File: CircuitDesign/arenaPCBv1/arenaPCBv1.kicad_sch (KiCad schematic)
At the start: 17 parts, among them Q1 IRF520N

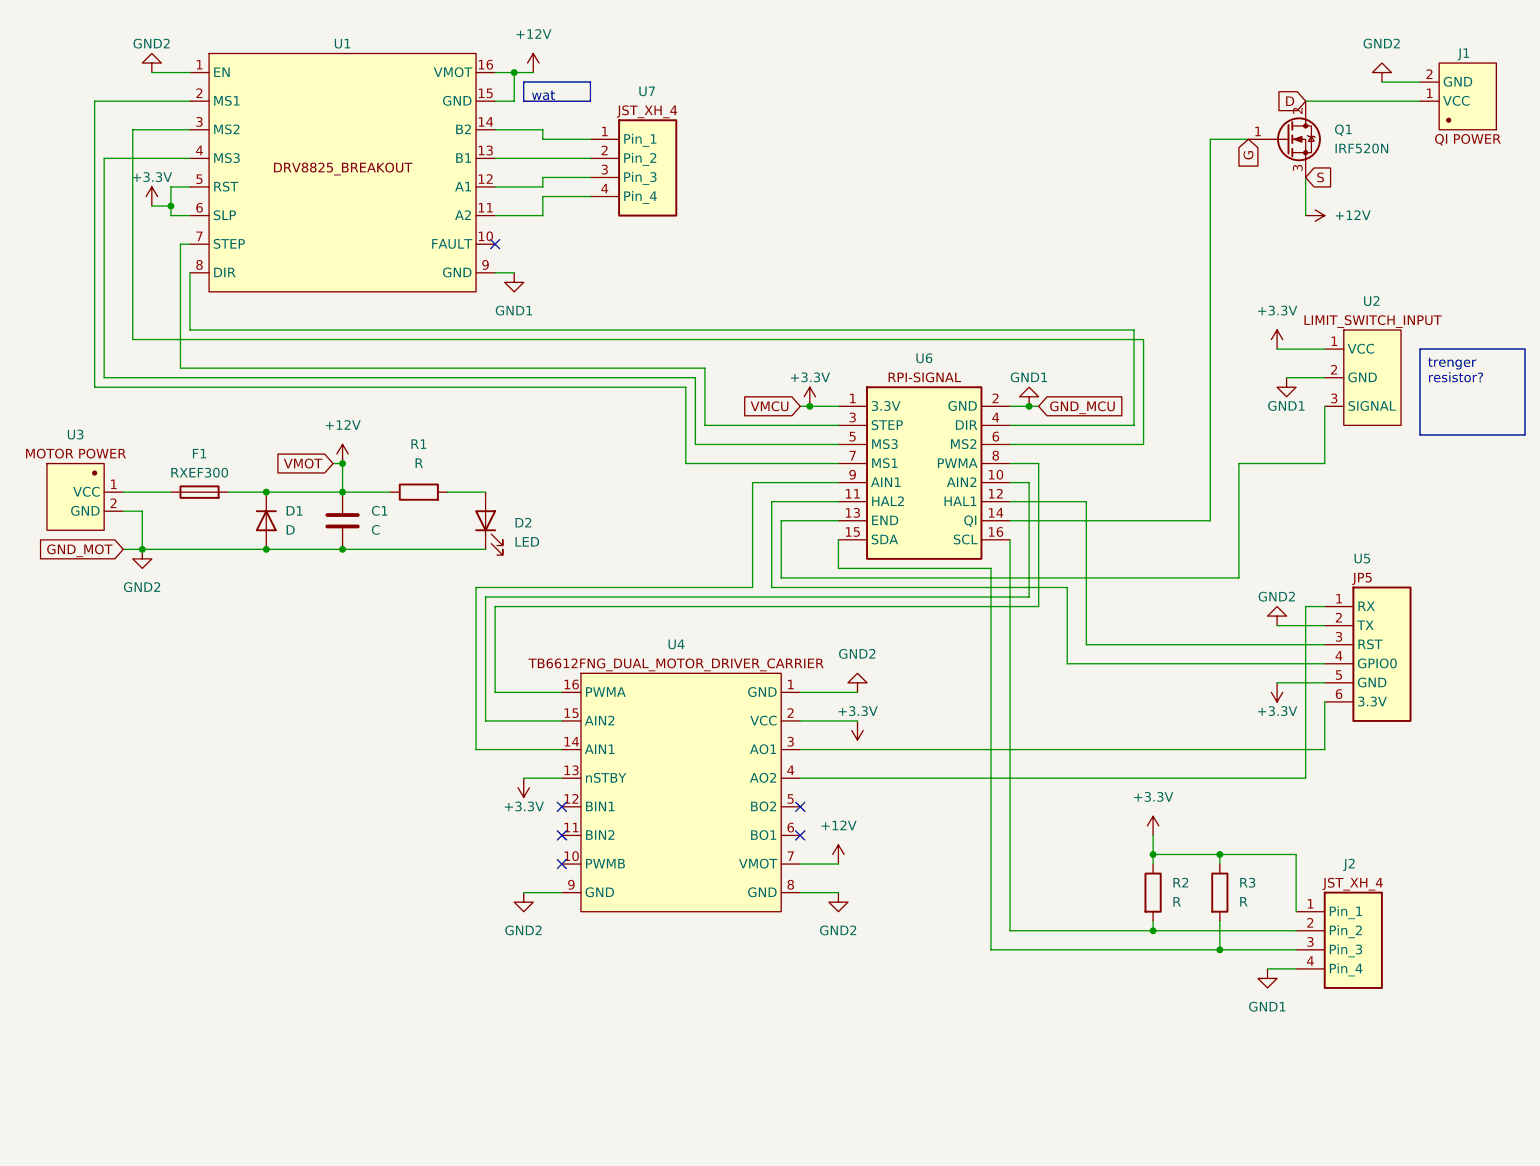
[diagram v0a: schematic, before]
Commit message: PCB v1 finished
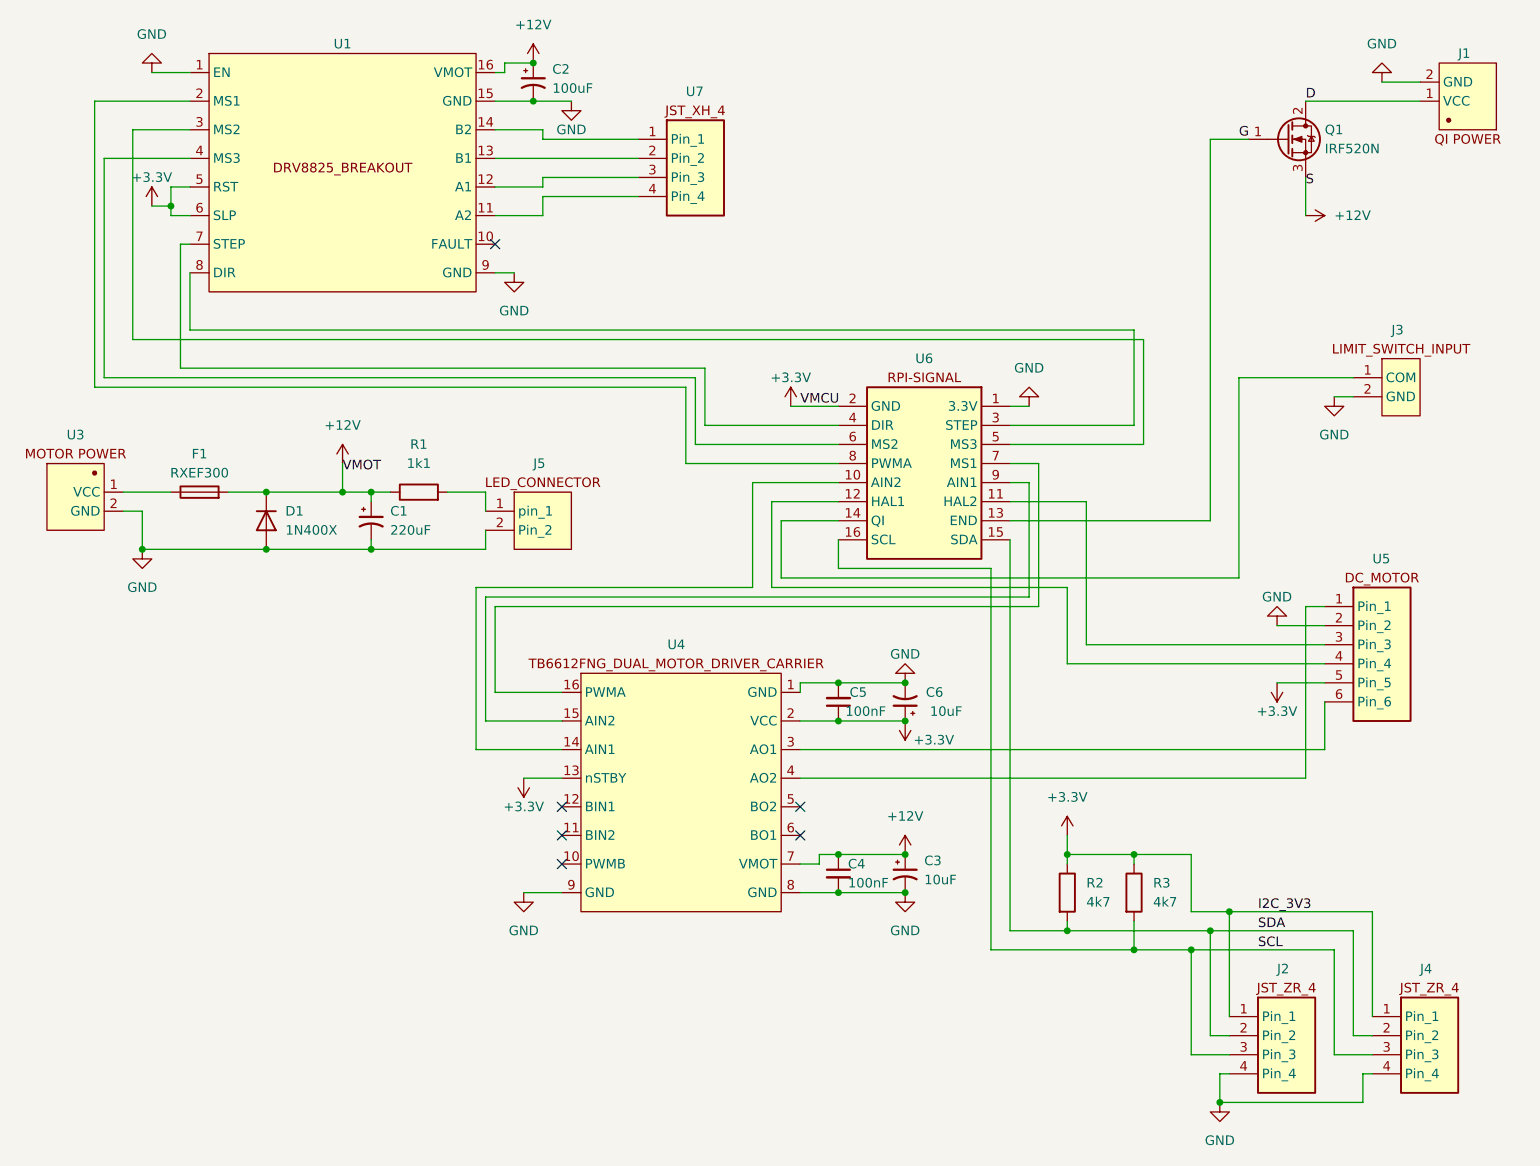
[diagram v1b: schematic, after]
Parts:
- removed C1: C, Capacitor_THT:CP_Radial_D13.0mm_P2.50mm, symbol Device:C
- removed D2: LED, LED_THT:LED_D3.0mm, symbol Device:LED
- removed U2: ~, Connector_PinHeader_1.27mm:PinHeader_1x03_P1.27mm_Vertical, symbol New_Library:Limit_Switch_Input
- added C1: 220uF, Capacitor_THT:CP_Radial_D10.0mm_P5.00mm, symbol Device:C_Polarized_Small_US
- added C2: 100uF, Capacitor_THT:CP_Radial_D8.0mm_P3.50mm, symbol Device:C_Polarized_Small_US
- added C3, C6: 10uF, Capacitor_THT:CP_Radial_D5.0mm_P2.00mm, symbol Device:C_Polarized_Small_US
- added C4, C5: 100nF, Capacitor_THT:C_Disc_D3.8mm_W2.6mm_P2.50mm, symbol Device:C_Small
- added J3: ~, Connector_JST:JST_PH_B2B-PH-K_1x02_P2.00mm_Vertical, symbol 1_Bachelors_Symbols:Limit_switch_input
- added J4: ~, Connector_JST:JST_PH_B4B-PH-K_1x04_P2.00mm_Vertical, symbol 1_Bachelors_Symbols:JST_VH_4
- added J5: ~, Connector_PinSocket_2.00mm:PinSocket_1x02_P2.00mm_Vertical, symbol 1_Bachelors_Symbols:LED_Connector
- D1: value D -> 1N400X
- J1: footprint (none) -> Connector_TE-Connectivity:TE_826576-2_1x02_P3.96mm_Vertical
- J2: footprint (none) -> Connector_JST:JST_PH_B4B-PH-K_1x04_P2.00mm_Vertical; symbol 1_Bachelors_Symbols:JST_XH_4 -> 1_Bachelors_Symbols:JST_VH_4
- R1: value R -> 1k1; footprint Resistor_THT:R_Axial_DIN0207_L6.3mm_D2.5mm_P10.16mm_Horizontal -> Resistor_THT:R_Axial_DIN0207_L6.3mm_D2.5mm_P15.24mm_Horizontal
- R2, R3: value R -> 4k7; footprint (none) -> Resistor_THT:R_Axial_DIN0207_L6.3mm_D2.5mm_P15.24mm_Horizontal
- U3: footprint Connector:JWT_A3963_1x02_P3.96mm_Vertical -> TerminalBlock_Phoenix:TerminalBlock_Phoenix_PT-1,5-2-3.5-H_1x02_P3.50mm_Horizontal
- U5: footprint Connector_PinHeader_1.27mm:PinHeader_1x06_P1.27mm_Vertical -> Connector_JST:JST_XH_B6B-XH-A_1x06_P2.50mm_Vertical
- U6: footprint Connector_PinHeader_1.00mm:PinHeader_2x08_P1.00mm_Vertical -> Connector_JST:JST_PHD_B16B-PHDSS_2x08_P2.00mm_Vertical
- U7: footprint Connector_PinHeader_1.27mm:PinHeader_1x04_P1.27mm_Vertical -> Connector_JST:JST_XH_B4B-XH-A_1x04_P2.50mm_Vertical
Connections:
- net GND2 is gone; now on net GND: D1.2 (A), J1.2 (GND), U1.1 (EN), U3.2 (GND), U4.1 (GND), U4.8 (GND), U4.9 (GND), U5.2 (Pin_2)
- net +12V: now also C1.1, C2.1, C3.1, C4.1; no longer U1.15 (GND)
- net +3.3V: now also U6.2 (GND), C5.1, C6.1, J4.1 (Pin_1); no longer U6.1 (3.3V)
- net G: now also U6.13 (END); no longer U6.14 (QI)
- net at R1.2: now also J5.1 (pin_1)
- net SDA: now reaches J2.2 (Pin_2), R2.2
- net SDA: now also U6.15 (SDA), J4.2 (Pin_2); no longer U6.16 (SCL)
- net SCL: now reaches J2.3 (Pin_3), R3.2
- net SCL: now also U6.16 (SCL), J4.3 (Pin_3); no longer U6.15 (SDA)
- net at U5.3 (Pin_3): now also U6.11 (HAL2); no longer U6.12 (HAL1)
- net at U5.4 (Pin_4): now also U6.12 (HAL1); no longer U6.11 (HAL2)
- net at U4.14 (AIN1): now also U6.10 (AIN2); no longer U6.9 (AIN1)
- net at U4.15 (AIN2): now also U6.9 (AIN1); no longer U6.10 (AIN2)
- net at U4.16 (PWMA): now also U6.7 (MS1); no longer U6.8 (PWMA)
- net at U1.2 (MS1): now also U6.8 (PWMA); no longer U6.7 (MS1)
- net at U1.3 (MS2): now also U6.5 (MS3); no longer U6.6 (MS2)
- net at U1.4 (MS3): now also U6.6 (MS2); no longer U6.5 (MS3)
- net at U1.7 (STEP): now also U6.4 (DIR); no longer U6.3 (STEP)
- net at U1.8 (DIR): now also U6.3 (STEP); no longer U6.4 (DIR)
- net GND1 renamed GND
- net GND: now also U1.15 (GND), U6.1 (3.3V), C1.2, C2.2, C3.2, C4.2, C5.2, C6.2, J3.2 (GND), J4.4 (Pin_4), J5.2 (Pin_2); no longer U6.2 (GND)
- new net: J3.1 (COM), U6.14 (QI)
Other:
- moved on the sheet: J2, R2, R3, U5, U7
